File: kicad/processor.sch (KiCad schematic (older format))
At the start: 18 parts, among them J2 Debug, J5 USB-C, Q2 AO3400A, U3 STM32L062K8Tx, U8 SRV05-4

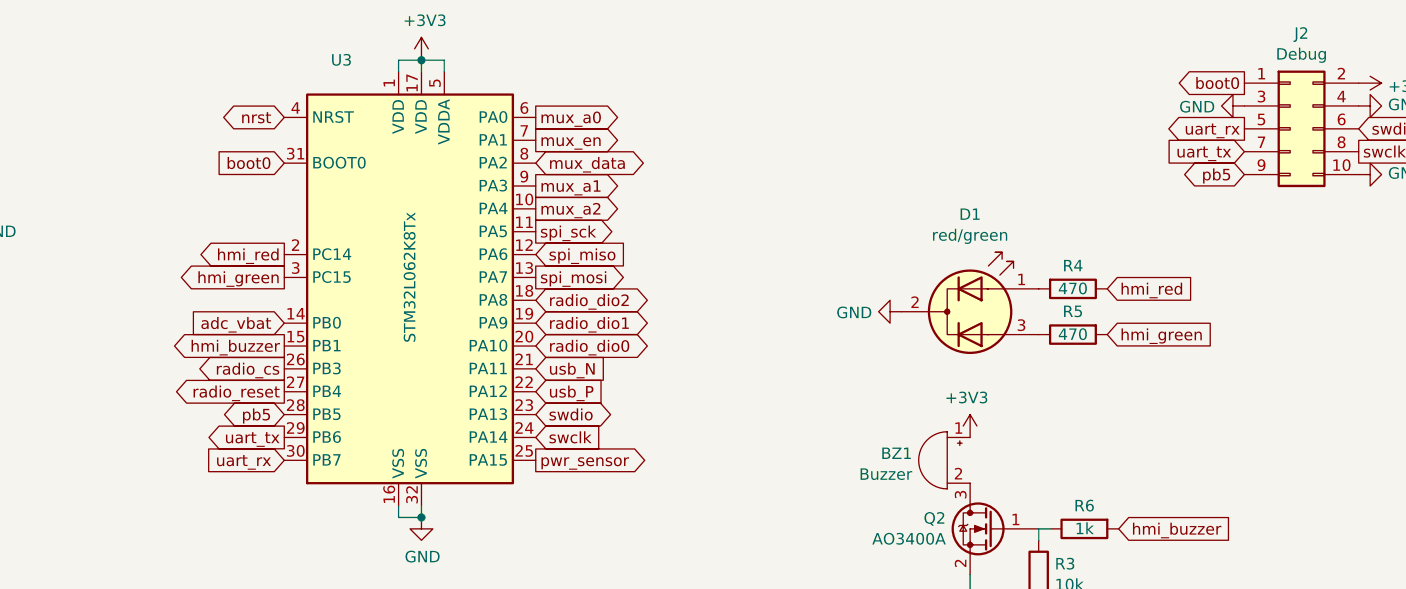
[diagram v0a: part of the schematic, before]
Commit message: lucy_v1.0
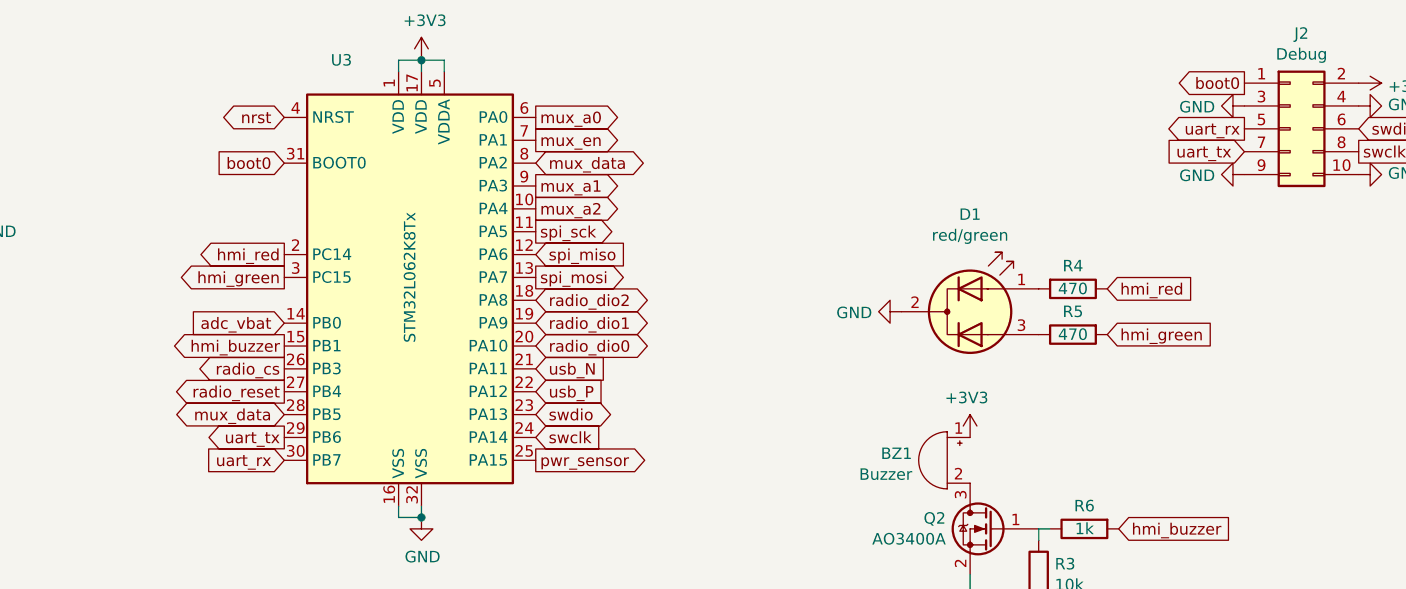
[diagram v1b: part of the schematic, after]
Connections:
- net GND: now also J2.9 (Pin_9)
- net mux_data: now also U3.28 (PB5)
- removed net pb5: J2.9 (Pin_9), U3.28 (PB5)
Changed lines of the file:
@@
 Sheet 3 5
 Title "Lucy"
-Date "2020-11-19"
+Date "2020-11-23"
 Rev "v1.0"
 Comp "www.2-0.dk"
@@
 Text GLabel 4050 3550 0    50   Output ~ 0
 hmi_red
-Text GLabel 8250 3200 0    50   BiDi ~ 0
-pb5
 Text GLabel 4050 3650 0    50   Output ~ 0
 hmi_green
-Text GLabel 4050 4250 0    50   BiDi ~ 0
-pb5
 $Comp
 L power:GND #PWR?
@@
 	1    0    0    -1
 $EndComp
+Text GLabel 4050 4250 0    50   BiDi ~ 0
+mux_data
+$Comp
+L power:GND #PWR?
+U 1 1 5FBD0670
+P 8250 3200
+AR Path="/5FBD0670" Ref="#PWR?"  Part="1"
+AR Path="/5E07BDE0/5FBD0670" Ref="#PWR02"  Part="1"
+F 0 "#PWR02" H 8250 2950 50  0001 C CNN
+F 1 "GND" V 8255 3072 50  0000 R CNN
+F 2 "" H 8250 3200 50  0001 C CNN
+F 3 "" H 8250 3200 50  0001 C CNN
+	1    8250 3200
+	0    1    1    0
+$EndComp
 $EndSCHEMATC
